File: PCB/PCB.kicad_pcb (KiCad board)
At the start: 2 copper layers, 222.6 x 128.5 mm, 78 parts, among them SW10 SW_Push, SW11 SW_Push, SW12 SW_Push, SW13 SW_Push, SW14 SW_Push, SW15 SW_Push, SW16 SW_Push, SW17 SW_Push, SW18 SW_Push, SW19 SW_Push, SW2 SW_Push, SW20 SW_Push, SW21 SW_Push, SW22 SW_Push, SW23 SW_Push, SW24 SW_Push, SW25 SW_Push, SW26 SW_Push, SW3 SW_Push, SW4 SW_Push, SW5 SW_Push, SW6 SW_Push, SW7 SW_Push, SW8 SW_Push, SW9 SW_Push, U1 COM-09032, U2 COM-09032

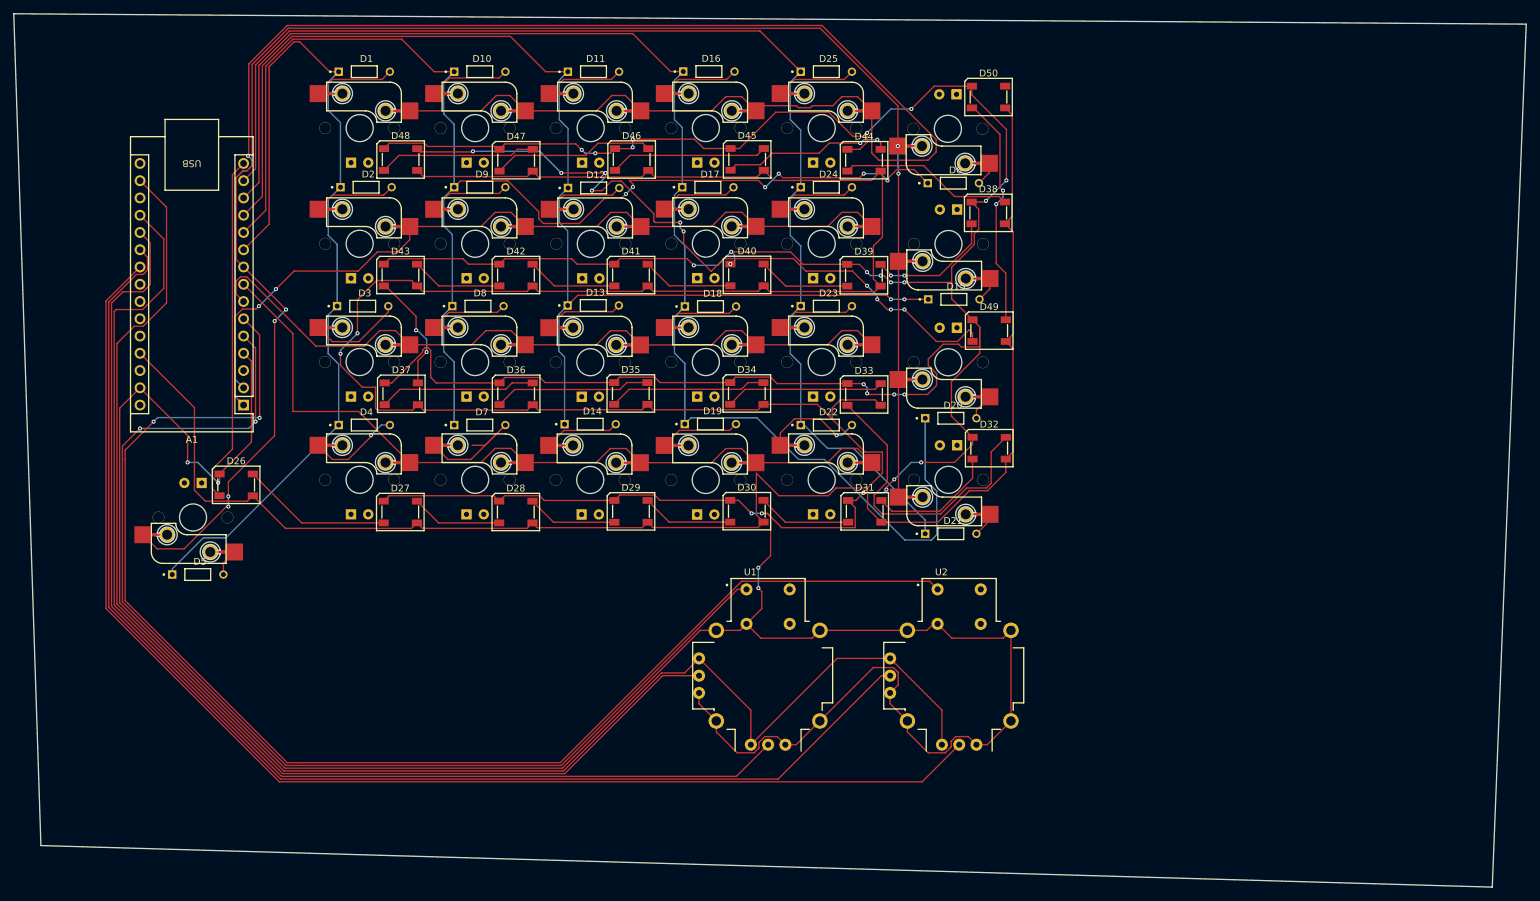
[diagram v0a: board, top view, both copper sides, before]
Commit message: get rid of lock files
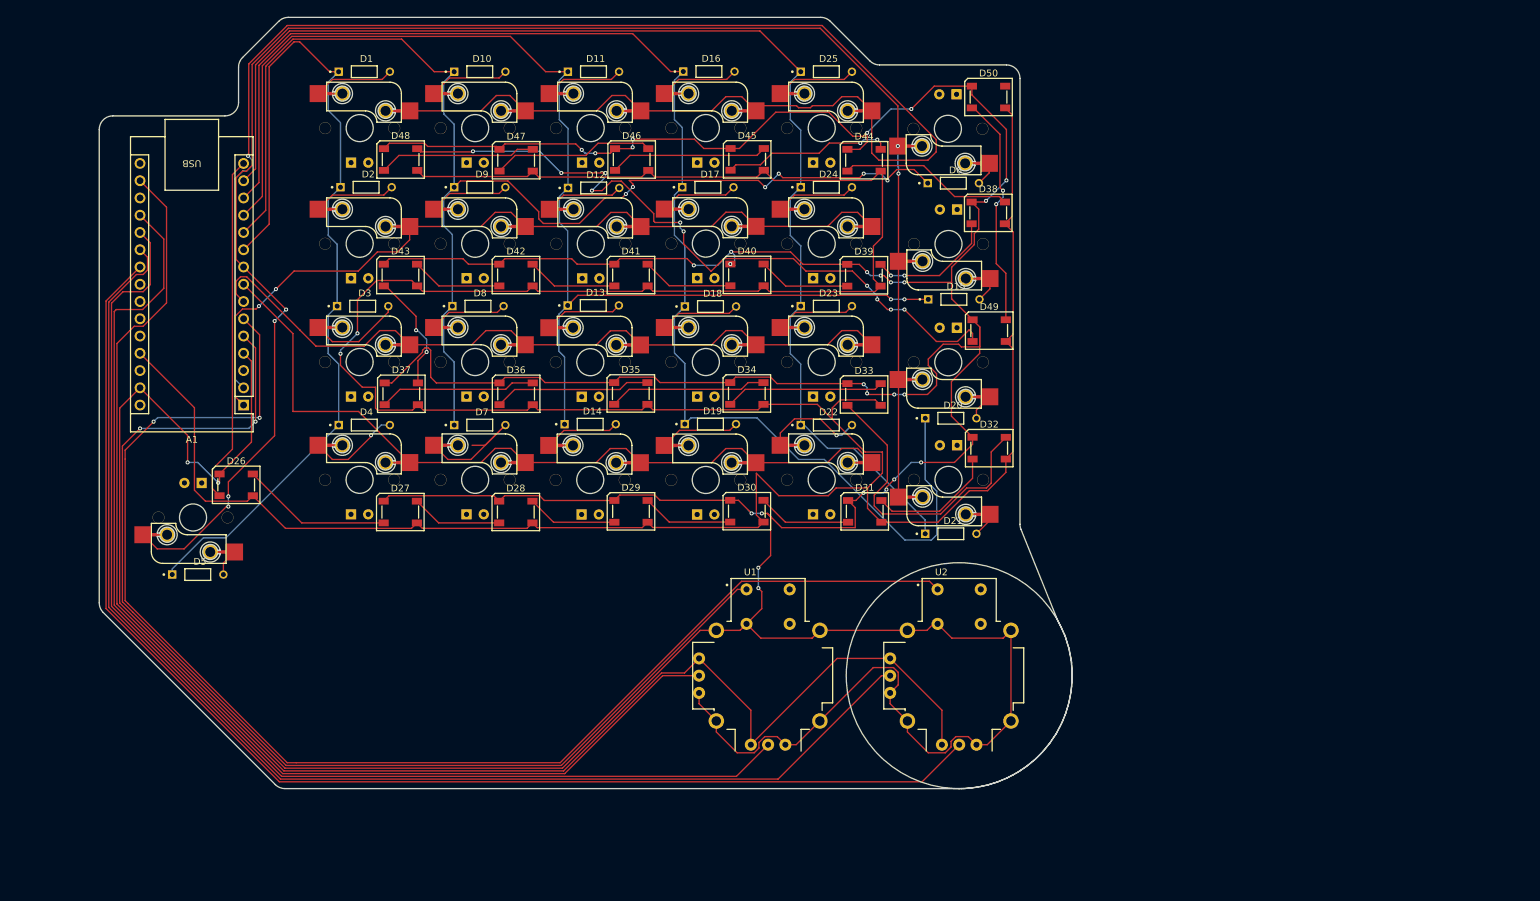
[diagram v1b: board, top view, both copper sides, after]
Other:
- board size 222.6 x 128.5 mm -> 143.2 x 113.5 mm
- board text added: "Made by @itsme with skill issues"
- board text added: "STNO"
